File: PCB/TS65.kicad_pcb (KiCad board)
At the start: 2 copper layers, 299.5 x 105.8 mm, 435 parts, among them P1 USB_CONN, P11 2PIN, P12 2PIN, P13 2PIN, P15 2PIN, P2 USB3, P3 USB3_MICRO, P4 6PIN, P5 6PIN, P6 ISP6, P7_1 5PIN, P7_2 5PIN, U1 Atmega32u4, U2 MCP23018, U3 IP4234CZ6, U4 74HC138, U5 PAM2804, X1 CRYSTAL

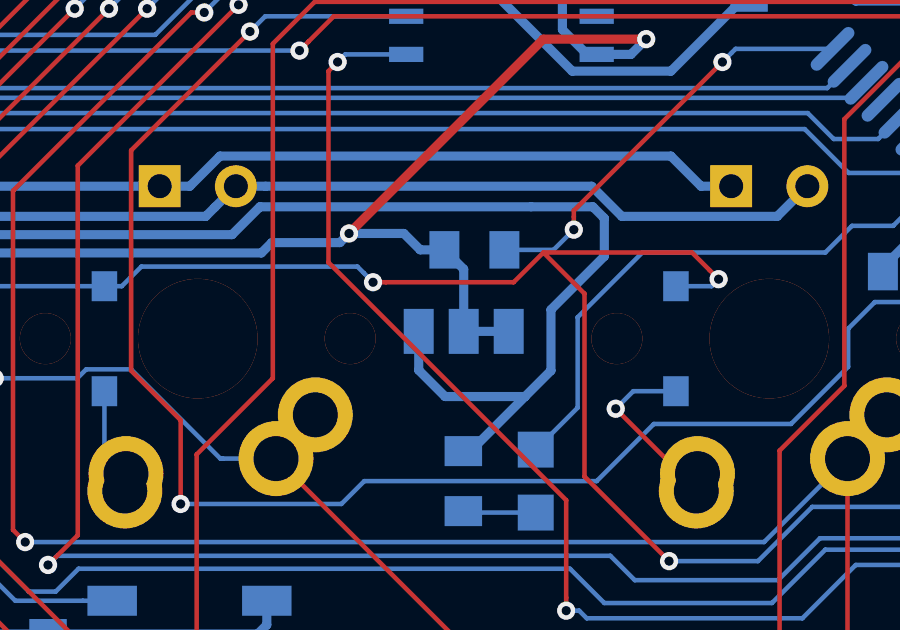
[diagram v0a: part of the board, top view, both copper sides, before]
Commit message: Rev 0.7
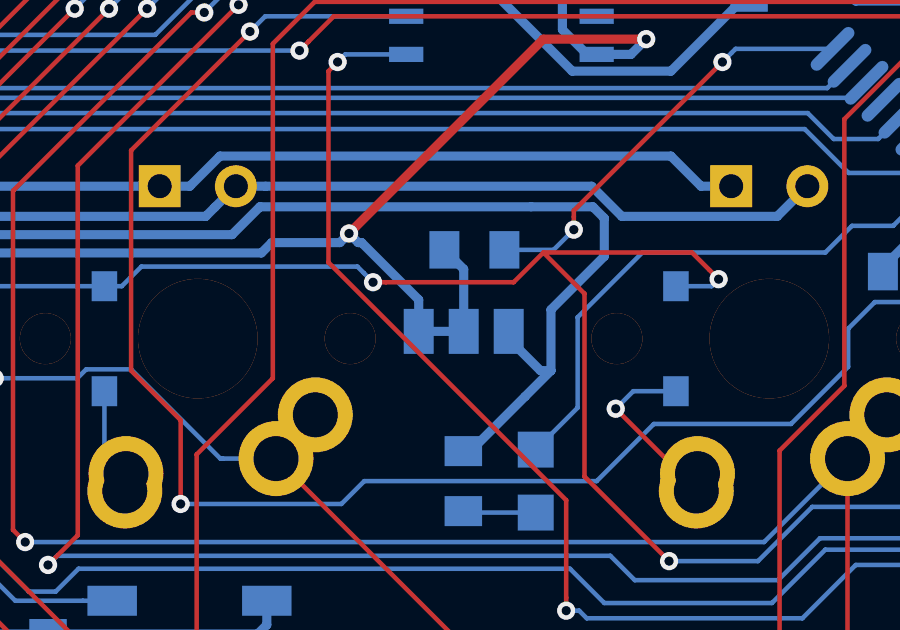
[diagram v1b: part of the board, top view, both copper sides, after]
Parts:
- turned JP1 to 180 degrees
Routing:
- net +5V: track 1279.5 -> 1276.4 mm
- net VSS: track 1175.8 -> 1176.6 mm
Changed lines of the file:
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@@
   )
   (module prettylib:JUMPER_SMD_3 (layer Back)
-    (at 135.1407 88.2269)
-    (fp_text reference JP1 (at 0.0635 1.8288) (layer B.SilkS)
+    (at 135.1407 88.2269 180)
+    (fp_text reference JP1 (at -0.1143 -1.8161 180) (layer B.SilkS)
       (effects (font (size 1 1) (thickness 0.25)) (justify mirror))
     )
-    (fp_text value JUMPER (at 0.254 -1.524) (layer Dwgs.User)
+    (fp_text value JUMPER (at 0.254 -1.524 180) (layer Dwgs.User)
       (effects (font (size 0.5 0.5) (thickness 0.1)))
     )
@@
     (fp_line (start 2.159 -1.016) (end -2.159 -1.016) (layer B.SilkS) (width 0.2))
     (fp_line (start -2.159 -1.016) (end -2.159 1.016) (layer B.SilkS) (width 0.2))
-    (pad 2 smd rect (at 0 0) (size 1 1.5) (layers Back B.Paste B.Mask)
+    (pad 2 smd rect (at 0 0 180) (size 1 1.5) (layers Back B.Paste B.Mask)
       (net 1 VSS))
-    (pad 1 smd rect (at -1.5 0 180) (size 1 1.5) (layers Back B.Paste B.Mask)
+    (pad 1 smd rect (at -1.5 0) (size 1 1.5) (layers Back B.Paste B.Mask)
       (net 68 +5V))
-    (pad 3 smd rect (at 1.5 0 180) (size 1 1.5) (layers Back B.Paste B.Mask)
+    (pad 3 smd rect (at 1.5 0) (size 1 1.5) (layers Back B.Paste B.Mask)
       (net 1 VSS))
   )
@@
   (gr_line (start 213.7 100.8) (end 205.8 100.8) (layer Edge.Cuts) (width 0.127))
   (gr_line (start 214.5 85.4) (end 214.5 100) (layer Edge.Cuts) (width 0.127))
-  (segment (start 136.6407 88.2269) (end 135.1407 88.2269) (width 0.3048) (layer Back) (net 1))
+  (segment (start 133.6407 88.2269) (end 135.1407 88.2269) (width 0.3048) (layer Back) (net 1))
+  (segment (start 133.6407 88.2269) (end 133.6407 87.1721) (width 0.3048) (layer Back) (net 1))
+  (segment (start 133.6407 87.1721) (end 131.736399 85.267799) (width 0.3048) (layer Back) (net 1))
+  (segment (start 131.736399 85.267799) (end 131.622799 85.267799) (width 0.3048) (layer Back) (net 1))
+  (segment (start 131.622799 85.267799) (end 131.318 84.963) (width 0.3048) (layer Back) (net 1))
   (segment (start 135.1407 88.2269) (end 135.1407 86.1535) (width 0.3048) (layer Back) (net 1))
   (segment (start 135.1407 86.1535) (end 134.4963 85.5091) (width 0.3048) (layer Back) (net 1))
-  (segment (start 131.749052 84.963) (end 131.318 84.963) (width 0.3048) (layer Back) (net 1))
-  (segment (start 133.1454 84.963) (end 131.749052 84.963) (width 0.3048) (layer Back) (net 1))
-  (segment (start 133.6915 85.5091) (end 133.1454 84.963) (width 0.3048) (layer Back) (net 1))
-  (segment (start 134.4963 85.5091) (end 133.6915 85.5091) (width 0.3048) (layer Back) (net 1))
   (segment (start 128.397 85.612212) (end 102.728788 85.612212) (width 0.3048) (layer Back) (net 1))
   (segment (start 131.318 84.963) (end 131.013201 85.267799) (width 0.3048) (layer Back) (net 1))
@@
   (segment (start 154.305 118.475) (end 162.420253 118.475) (width 0.1524) (layer Back) (net 67))
   (segment (start 162.420253 118.475) (end 164.338 120.392747) (width 0.1524) (layer Back) (net 67))
-  (segment (start 133.6407 88.2269) (end 133.6407 89.5209) (width 0.3048) (layer Back) (net 68))
-  (segment (start 134.5184 90.3986) (end 137.1854 90.3986) (width 0.3048) (layer Back) (net 68))
-  (segment (start 133.6407 89.5209) (end 134.5184 90.3986) (width 0.3048) (layer Back) (net 68))
+  (segment (start 138.049 89.535) (end 137.6988 89.535) (width 0.3048) (layer Back) (net 68))
+  (segment (start 137.6988 89.535) (end 136.6407 88.4769) (width 0.3048) (layer Back) (net 68))
+  (segment (start 136.6407 88.4769) (end 136.6407 88.2269) (width 0.3048) (layer Back) (net 68))
   (segment (start 135.366 92.218) (end 137.1854 90.3986) (width 0.3048) (layer Back) (net 68))
   (segment (start 137.1854 90.3986) (end 138.049 89.535) (width 0.3048) (layer Back) (net 68))
@@
       )
     )
+  )
+  (zone (net 0) (net_name "") (layer Back) (hatch edge 0.508)
+    (connect_pads (clearance 0.308))
+    (min_thickness 0.254)
+    (keepout (tracks allowed) (vias allowed) (copperpour not_allowed))
+    (fill (arc_segments 16) (thermal_gap 0.508) (thermal_bridge_width 0.508))
+    (polygon
+      (pts
+        (xy 133.096 89.408) (xy 137.16 89.408) (xy 137.16 84.328) (xy 133.096 84.328)
+      )
+    )
